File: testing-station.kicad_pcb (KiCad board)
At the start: 4 copper layers, 176.5 x 77.1 mm, 2 parts, among them J11 FPC connector

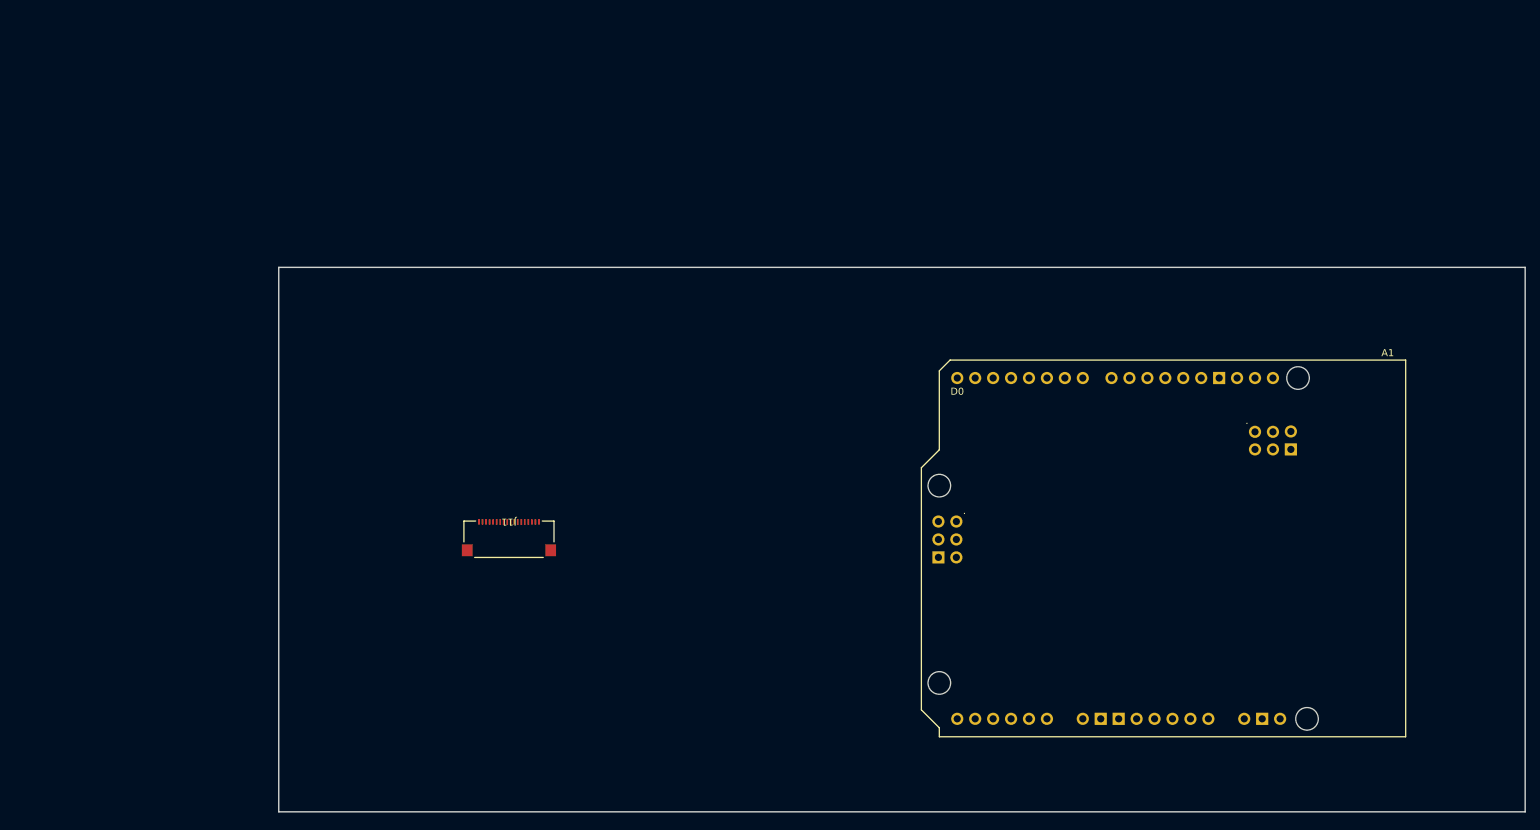
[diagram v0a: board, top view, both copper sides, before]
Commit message: added PCB layout
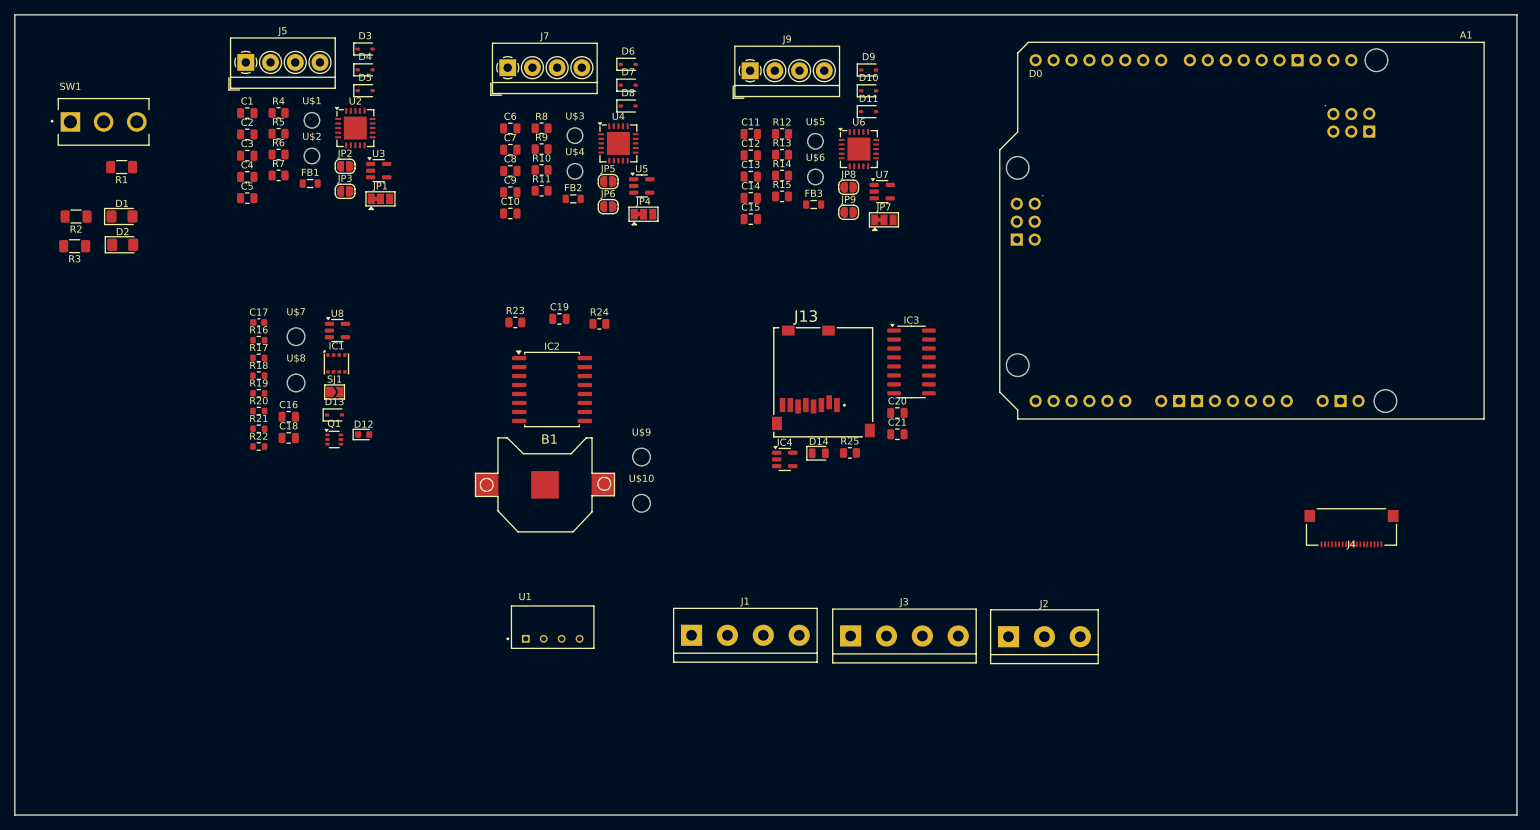
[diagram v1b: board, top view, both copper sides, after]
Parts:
- removed J11: FPC connector, external_footprints:XF2M-1815-1A
- added B1: CR1220, external_footprints:CR1220, F.Cu at (116.7, 88.1)
- added C1: 0.1uF, Capacitor_SMD:C_0805_2012Metric, F.Cu at (74.5, 35.5)
- added C10: 10uF, Capacitor_SMD:C_0805_2012Metric, F.Cu at (111.8, 49.7)
- added C11: 0.1uF, Capacitor_SMD:C_0805_2012Metric, F.Cu at (145.8, 38.4)
- added C12: 0.1uF, Capacitor_SMD:C_0805_2012Metric, F.Cu at (145.8, 41.4)
- added C13: 0.1uF, Capacitor_SMD:C_0805_2012Metric, F.Cu at (145.8, 44.5)
- added C14: 10uF, Capacitor_SMD:C_0805_2012Metric, F.Cu at (145.8, 47.5)
- added C15: 10uF, Capacitor_SMD:C_0805_2012Metric, F.Cu at (145.8, 50.5)
- added C16: 10uF, Capacitor_SMD:C_0805_2012Metric, F.Cu at (80.4, 78.5)
- added C17: 0.1uF, Capacitor_SMD:C_0603_1608Metric, F.Cu at (76.2, 65.1)
- added C18: 10uF, Capacitor_SMD:C_0805_2012Metric, F.Cu at (80.4, 81.5)
- added C19: 1uF, Capacitor_SMD:C_0805_2012Metric, F.Cu at (118.8, 64.6)
- added C2: 0.1uF, Capacitor_SMD:C_0805_2012Metric, F.Cu at (74.5, 38.5)
- added C20: 10uF, Capacitor_SMD:C_0805_2012Metric, F.Cu at (166.6, 77.9)
- added C21: 0.1uF, Capacitor_SMD:C_0805_2012Metric, F.Cu at (166.6, 80.9)
- added C3: 0.1uF, Capacitor_SMD:C_0805_2012Metric, F.Cu at (74.5, 41.5)
- added C4: 10uF, Capacitor_SMD:C_0805_2012Metric, F.Cu at (74.5, 44.5)
- added C5: 10uF, Capacitor_SMD:C_0805_2012Metric, F.Cu at (74.5, 47.5)
- added C6: 0.1uF, Capacitor_SMD:C_0805_2012Metric, F.Cu at (111.8, 37.6)
- added C7: 0.1uF, Capacitor_SMD:C_0805_2012Metric, F.Cu at (111.8, 40.6)
- added C8: 0.1uF, Capacitor_SMD:C_0805_2012Metric, F.Cu at (111.8, 43.6)
- added C9: 10uF, Capacitor_SMD:C_0805_2012Metric, F.Cu at (111.8, 46.7)
- added D1: LED_GREEN, LED_SMD:LED_1206_3216Metric_Pad1.42x1.75mm_HandSolder, F.Cu at (56.8, 50.1)
- added D10: 1N4148, Diode_SMD:D_SOD-323, F.Cu at (162.5, 32.3)
- added D11: 1N4148, Diode_SMD:D_SOD-323, F.Cu at (162.5, 35.2)
- added D12: GREEN, LED_SMD:LED_0603_1608Metric, F.Cu at (91.0, 81.0)
- added D13: 1N4148, Diode_SMD:D_SOD-323, F.Cu at (86.9, 78.2)
- added D14: RED, LED_SMD:LED_0805_2012Metric, F.Cu at (155.5, 83.6)
- added D2: LED_RED, LED_SMD:LED_1206_3216Metric_Pad1.42x1.75mm_HandSolder, F.Cu at (56.9, 54.1)
- added D3: 1N4148, Diode_SMD:D_SOD-323, F.Cu at (91.2, 26.4)
- added D4: 1N4148, Diode_SMD:D_SOD-323, F.Cu at (91.2, 29.3)
- added D5: 1N4148, Diode_SMD:D_SOD-323, F.Cu at (91.2, 32.3)
- added D6: 1N4148, Diode_SMD:D_SOD-323, F.Cu at (128.5, 28.6)
- added D7: 1N4148, Diode_SMD:D_SOD-323, F.Cu at (128.5, 31.5)
- added D8: 1N4148, Diode_SMD:D_SOD-323, F.Cu at (128.5, 34.5)
- added D9: 1N4148, Diode_SMD:D_SOD-323, F.Cu at (162.5, 29.4)
- added FB1: FERRITE-0805NO, Inductor_SMD:L_0805_2012Metric, F.Cu at (83.5, 45.4)
- added FB2: FERRITE-0805NO, Inductor_SMD:L_0805_2012Metric, F.Cu at (120.7, 47.6)
- added FB3: FERRITE-0805NO, Inductor_SMD:L_0805_2012Metric, F.Cu at (154.8, 48.4)
- added IC1: BME680, Package_LGA:Bosch_LGA-8_3x3mm_P0.8mm_ClockwisePinNumbering, F.Cu at (87.2, 70.9)
- added IC2: DS3231, Package_SO:SOIC-16W_7.5x10.3mm_P1.27mm, F.Cu at (117.7, 74.6)
- added IC3: 74HC4050D, Package_SO:SOIC-16_3.9x9.9mm_P1.27mm, F.Cu at (168.6, 70.7)
- added IC4: LP2985A, Package_TO_SOT_SMD:SOT-23-5, F.Cu at (150.7, 84.5)
- added J1: pyranometer, TerminalBlock:TerminalBlock_bornier-4_P5.08mm, F.Cu at (137.5, 109.4)
- added J13: microSD, external_footprints:MEM2061-01-188-00-A, F.Cu at (156.1, 73.6)
- added J2: anemometer, TerminalBlock:TerminalBlock_bornier-3_P5.08mm, F.Cu at (182.3, 109.6)
- added J3: AM2315C, TerminalBlock:TerminalBlock_bornier-4_P5.08mm, F.Cu at (160.0, 109.5)
- added J4: FPC connector, external_footprints:XF2M-1815-1A, F.Cu at (230.9, 94.1)
- added J5: Pt100, TerminalBlock_4Ucon:TerminalBlock_4Ucon_1x04_P3.50mm_Horizontal, F.Cu at (74.3, 28.3)
- added J7: Pt100, TerminalBlock_4Ucon:TerminalBlock_4Ucon_1x04_P3.50mm_Horizontal, F.Cu at (111.4, 29.0)
- added J9: Pt100, TerminalBlock_4Ucon:TerminalBlock_4Ucon_1x04_P3.50mm_Horizontal, F.Cu at (145.8, 29.4)
- added JP1: SolderJumper_3_Bridged12, Jumper:SolderJumper-3_P1.3mm_Bridged12_Pad1.0x1.5mm, F.Cu at (93.4, 47.6)
- added JP2: SOLDERJUMPER, Jumper:SolderJumper-2_P1.3mm_Open_RoundedPad1.0x1.5mm, F.Cu at (88.4, 43.0)
- added JP3: SOLDERJUMPER, Jumper:SolderJumper-2_P1.3mm_Open_RoundedPad1.0x1.5mm, F.Cu at (88.4, 46.5)
- added JP4: SolderJumper_3_Bridged12, Jumper:SolderJumper-3_P1.3mm_Bridged12_Pad1.0x1.5mm, F.Cu at (130.7, 49.8)
- added JP5: SOLDERJUMPER, Jumper:SolderJumper-2_P1.3mm_Open_RoundedPad1.0x1.5mm, F.Cu at (125.7, 45.1)
- added JP6: SOLDERJUMPER, Jumper:SolderJumper-2_P1.3mm_Open_RoundedPad1.0x1.5mm, F.Cu at (125.7, 48.7)
- added JP7: SolderJumper_3_Bridged12, Jumper:SolderJumper-3_P1.3mm_Bridged12_Pad1.0x1.5mm, F.Cu at (164.7, 50.6)
- added JP8: SOLDERJUMPER, Jumper:SolderJumper-2_P1.3mm_Open_RoundedPad1.0x1.5mm, F.Cu at (159.7, 46.0)
- added JP9: SOLDERJUMPER, Jumper:SolderJumper-2_P1.3mm_Open_RoundedPad1.0x1.5mm, F.Cu at (159.7, 49.5)
- added Q1: BSS138, Package_TO_SOT_SMD:SOT-363_SC-70-6, F.Cu at (86.9, 81.7)
- added R1: 10k, Resistor_SMD:R_1206_3216Metric_Pad1.30x1.75mm_HandSolder, F.Cu at (56.8, 43.1)
- added R10: 10K, Resistor_SMD:R_0805_2012Metric, F.Cu at (116.2, 43.5)
- added R11: 430Ω, ±0.1%, Resistor_SMD:R_0805_2012Metric, F.Cu at (116.2, 46.5)
- added R12: 10K, Resistor_SMD:R_0805_2012Metric, F.Cu at (150.3, 38.4)
- added R13: 10K, Resistor_SMD:R_0805_2012Metric, F.Cu at (150.3, 41.4)
- added R14: 10K, Resistor_SMD:R_0805_2012Metric, F.Cu at (150.3, 44.3)
- added R15: 430Ω, ±0.1%, Resistor_SMD:R_0805_2012Metric, F.Cu at (150.3, 47.2)
- added R16: 10k, Resistor_SMD:R_0603_1608Metric, F.Cu at (76.2, 67.6)
- added R17: 10k, Resistor_SMD:R_0603_1608Metric, F.Cu at (76.2, 70.1)
- added R18: 10k, Resistor_SMD:R_0603_1608Metric, F.Cu at (76.2, 72.6)
- added R19: 10k, Resistor_SMD:R_0603_1608Metric, F.Cu at (76.2, 75.1)
- added R2: 150, Resistor_SMD:R_1206_3216Metric_Pad1.30x1.75mm_HandSolder, F.Cu at (50.3, 50.1)
- added R20: 10k, Resistor_SMD:R_0603_1608Metric, F.Cu at (76.2, 77.7)
- added R21: 10k, Resistor_SMD:R_0603_1608Metric, F.Cu at (76.2, 80.2)
- added R22: 10k, Resistor_SMD:R_0603_1608Metric, F.Cu at (76.2, 82.7)
- added R23: 10k, Resistor_SMD:R_0805_2012Metric, F.Cu at (112.5, 65.1)
- added R24: 10k, Resistor_SMD:R_0805_2012Metric, F.Cu at (124.4, 65.3)
- added R25: 1k, Resistor_SMD:R_0805_2012Metric, F.Cu at (159.9, 83.6)
- added R3: 150, Resistor_SMD:R_1206_3216Metric_Pad1.30x1.75mm_HandSolder, F.Cu at (50.1, 54.3)
- added R4: 10K, Resistor_SMD:R_0805_2012Metric, F.Cu at (79.0, 35.4)
- added R5: 10K, Resistor_SMD:R_0805_2012Metric, F.Cu at (79.0, 38.4)
- added R6: 10K, Resistor_SMD:R_0805_2012Metric, F.Cu at (79.0, 41.3)
- added R7: 430Ω, ±0.1%, Resistor_SMD:R_0805_2012Metric, F.Cu at (79.0, 44.3)
- added R8: 10K, Resistor_SMD:R_0805_2012Metric, F.Cu at (116.2, 37.6)
- added R9: 10K, Resistor_SMD:R_0805_2012Metric, F.Cu at (116.2, 40.5)
- added SJ1: SOLDERJUMPER, Jumper:SolderJumper-2_P1.3mm_Open_TrianglePad1.0x1.5mm, F.Cu at (86.9, 75.0)
- added SW1: 500SSP1S2M2QEA, external_footprints:500SSP1S2M2QEA, F.Cu at (54.2, 36.7)
- added U$1: MOUNTINGHOLE2.5, MountingHole:MountingHole_2.2mm_M2_ISO7380, F.Cu at (83.7, 36.5)
- added U$10: MOUNTINGHOLE2.5, MountingHole:MountingHole_2.5mm, F.Cu at (130.4, 90.7)
- added U$2: MOUNTINGHOLE2.5, MountingHole:MountingHole_2.2mm_M2_ISO7380, F.Cu at (83.7, 41.5)
- added U$3: MOUNTINGHOLE2.5, MountingHole:MountingHole_2.2mm_M2_ISO7380, F.Cu at (121.0, 38.6)
- added U$4: MOUNTINGHOLE2.5, MountingHole:MountingHole_2.2mm_M2_ISO7380, F.Cu at (121.0, 43.7)
- added U$5: MOUNTINGHOLE2.5, MountingHole:MountingHole_2.2mm_M2_ISO7380, F.Cu at (155.0, 39.5)
- added U$6: MOUNTINGHOLE2.5, MountingHole:MountingHole_2.2mm_M2_ISO7380, F.Cu at (155.0, 44.5)
- added U$7: MOUNTINGHOLE2.5, MountingHole:MountingHole_2.5mm, F.Cu at (81.5, 67.1)
- added U$8: MOUNTINGHOLE2.5, MountingHole:MountingHole_2.5mm, F.Cu at (81.5, 73.7)
- added U$9: MOUNTINGHOLE2.5, MountingHole:MountingHole_2.5mm, F.Cu at (130.4, 84.2)
- added U1: TBA_1-0519, external_footprints:TBA_1-0519, F.Cu at (117.8, 108.2)
- added U2: MAX31865, Package_DFN_QFN:TQFN-20-1EP_5x5mm_P0.65mm_EP3.25x3.25mm, F.Cu at (89.8, 37.6)
- added U3: MIC5225, Package_TO_SOT_SMD:SOT-23-5, F.Cu at (93.2, 43.6)
- added U4: MAX31865, Package_DFN_QFN:TQFN-20-1EP_5x5mm_P0.65mm_EP3.25x3.25mm, F.Cu at (127.1, 39.8)
- added U5: MIC5225, Package_TO_SOT_SMD:SOT-23-5, F.Cu at (130.4, 45.8)
- added U6: MAX31865, Package_DFN_QFN:TQFN-20-1EP_5x5mm_P0.65mm_EP3.25x3.25mm, F.Cu at (161.2, 40.5)
- added U7: MIC5225, Package_TO_SOT_SMD:SOT-23-5, F.Cu at (164.4, 46.6)
- added U8: AP2112K-3.3, Package_TO_SOT_SMD:SOT-23-5, F.Cu at (87.3, 66.2)
- moved A1 46.3 mm to (249.7, 78.8)
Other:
- board size 176.5 x 77.1 mm -> 212.7 x 113.3 mm
